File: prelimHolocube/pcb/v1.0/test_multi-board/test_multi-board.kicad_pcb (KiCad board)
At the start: 2 copper layers, 120 x 100 mm, 4 parts

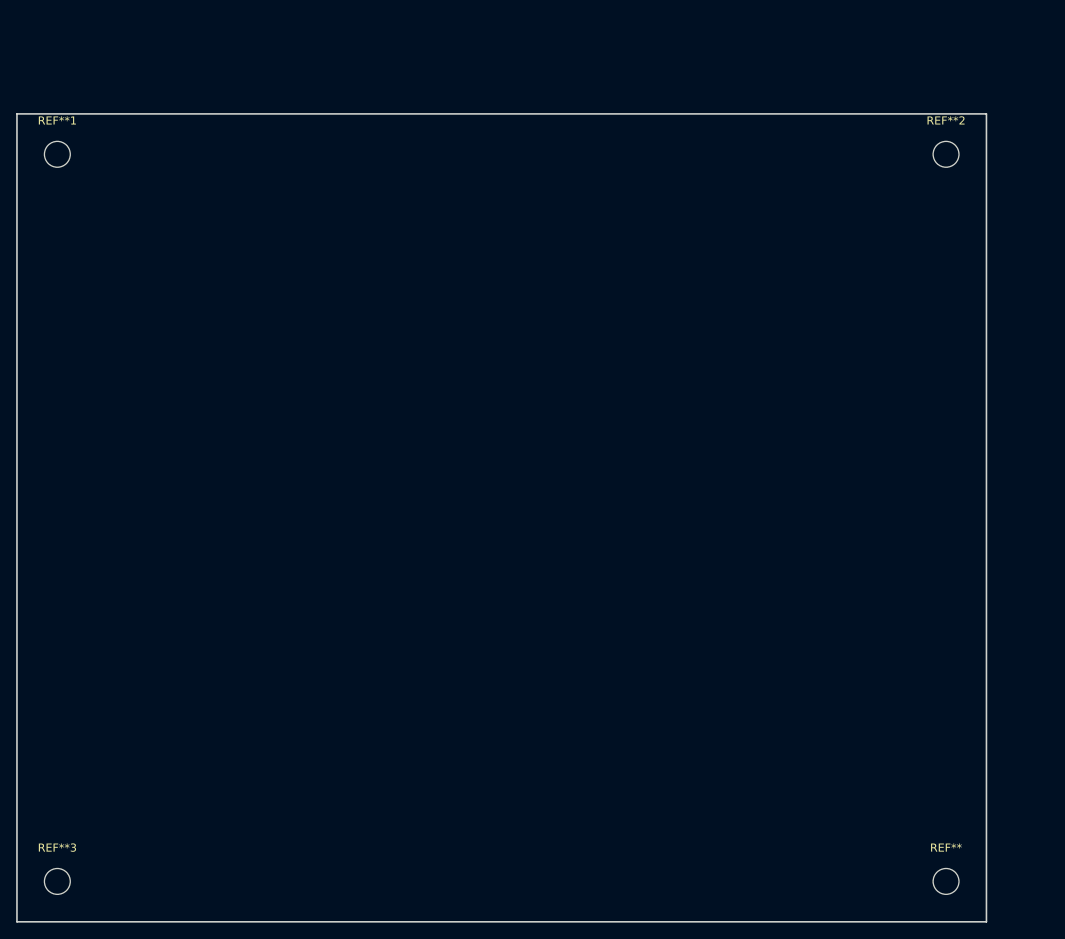
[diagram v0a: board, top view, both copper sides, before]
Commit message: Finish multiboard pcb
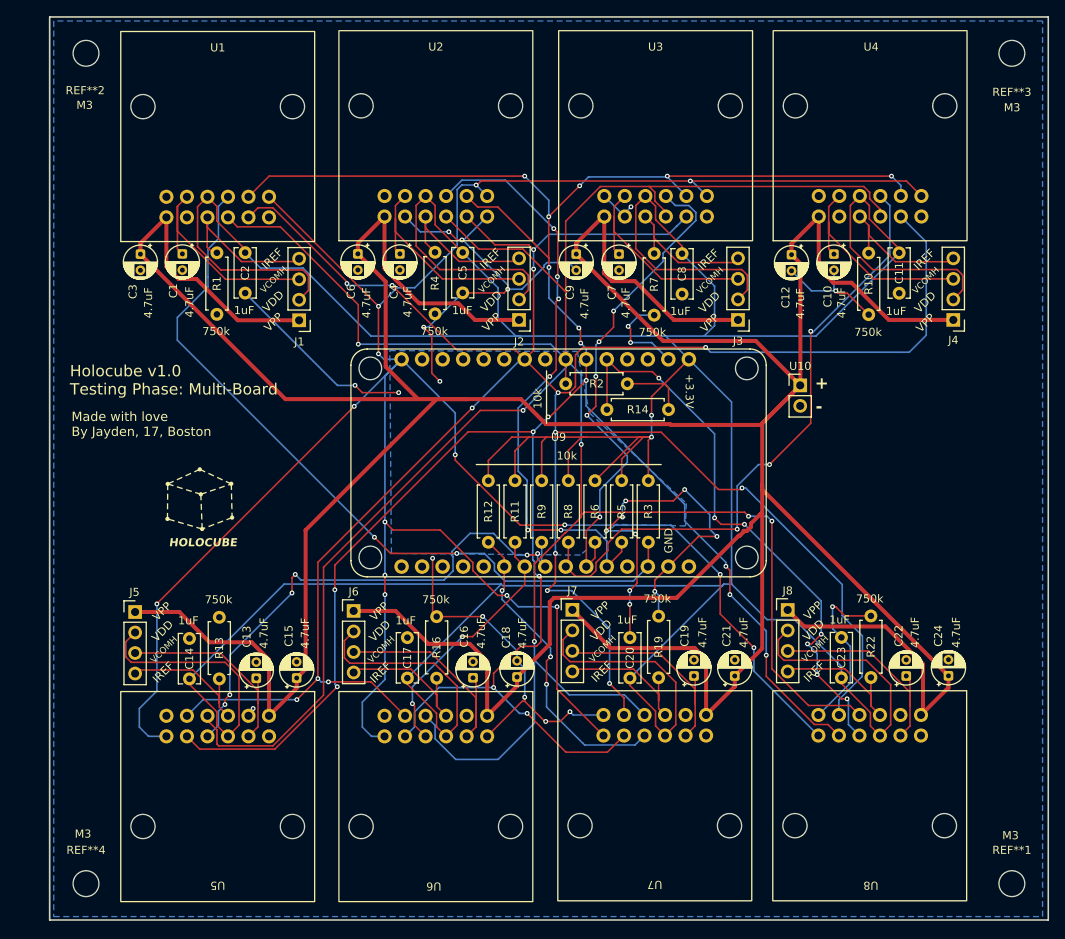
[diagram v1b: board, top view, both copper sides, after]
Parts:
- removed REF**: MountingHole_3.2mm_M3, MountingHole:MountingHole_3.2mm_M3
- added C1: 4.7uF, Capacitor_THT:CP_Radial_D4.0mm_P2.00mm, F.Cu at (109.9, 69.6)
- added C10: 4.7uF, Capacitor_THT:CP_Radial_D4.0mm_P2.00mm, F.Cu at (190.6, 69.7)
- added C11: 1uF ceramic, Capacitor_THT:C_Disc_D6.0mm_W2.5mm_P5.00mm, F.Cu at (198.7, 74.5)
- added C12: 4.7uF, Capacitor_THT:CP_Radial_D4.0mm_P2.00mm, F.Cu at (185.3, 69.7)
- added C13: 4.7uF, Capacitor_THT:CP_Radial_D4.0mm_P2.00mm, F.Cu at (119.1, 122.2)
- added C14: 1uF ceramic, Capacitor_THT:C_Disc_D6.0mm_W2.5mm_P5.00mm, F.Cu at (110.8, 117.2)
- added C15: 4.7uF, Capacitor_THT:CP_Radial_D4.0mm_P2.00mm, F.Cu at (124.1, 122.1)
- added C16: 4.7uF, Capacitor_THT:CP_Radial_D4.0mm_P2.00mm, F.Cu at (145.9, 122.1)
- added C17: 1uF ceramic, Capacitor_THT:C_Disc_D6.0mm_W2.5mm_P5.00mm, F.Cu at (137.8, 117.1)
- added C18: 4.7uF, Capacitor_THT:CP_Radial_D4.0mm_P2.00mm, F.Cu at (151.3, 122.0)
- added C19: 4.7uF, Capacitor_THT:CP_Radial_D4.0mm_P2.00mm, F.Cu at (173.2, 121.9)
- added C2: 1uF ceramic, Capacitor_THT:C_Disc_D6.0mm_W2.5mm_P5.00mm, F.Cu at (117.7, 74.5)
- added C20: 1uF ceramic, Capacitor_THT:C_Disc_D6.0mm_W2.5mm_P5.00mm, F.Cu at (165.3, 117.1)
- added C21: 4.7uF, Capacitor_THT:CP_Radial_D4.0mm_P2.00mm, F.Cu at (178.3, 121.9)
- added C22: 4.7uF, Capacitor_THT:CP_Radial_D4.0mm_P2.00mm, F.Cu at (199.5, 121.9)
- added C23: 1uF ceramic, Capacitor_THT:C_Disc_D6.0mm_W2.5mm_P5.00mm, F.Cu at (191.5, 117.1)
- added C24: 4.7uF, Capacitor_THT:CP_Radial_D4.0mm_P2.00mm, F.Cu at (204.8, 121.8)
- added C3: 4.7uF, Capacitor_THT:CP_Radial_D4.0mm_P2.00mm, F.Cu at (104.7, 69.7)
- added C4: 4.7uF, Capacitor_THT:CP_Radial_D4.0mm_P2.00mm, F.Cu at (136.8, 69.6)
- added C5: 1uF ceramic, Capacitor_THT:C_Disc_D6.0mm_W2.5mm_P5.00mm, F.Cu at (144.6, 74.5)
- added C6: 4.7uF, Capacitor_THT:CP_Radial_D4.0mm_P2.00mm, F.Cu at (131.7, 69.6)
- added C7: 4.7uF, Capacitor_THT:CP_Radial_D4.0mm_P2.00mm, F.Cu at (164.0, 69.7)
- added C8: 1uF ceramic, Capacitor_THT:C_Disc_D6.0mm_W2.5mm_P5.00mm, F.Cu at (171.8, 74.6)
- added C9: 4.7uF, Capacitor_THT:CP_Radial_D4.0mm_P2.00mm, F.Cu at (158.7, 69.7)
- added J1: Breakout_1, Connector_PinHeader_2.54mm:PinHeader_1x04_P2.54mm_Vertical, F.Cu at (124.4, 77.8)
- added J2: Breakout_2, Connector_PinHeader_2.54mm:PinHeader_1x04_P2.54mm_Vertical, F.Cu at (151.6, 77.8)
- added J3: Breakout_3, Connector_PinHeader_2.54mm:PinHeader_1x04_P2.54mm_Vertical, F.Cu at (178.7, 77.8)
- added J4: Breakout_4, Connector_PinHeader_2.54mm:PinHeader_1x04_P2.54mm_Vertical, F.Cu at (205.3, 77.8)
- added J5: Breakout_5, Connector_PinHeader_2.54mm:PinHeader_1x04_P2.54mm_Vertical, F.Cu at (104.1, 114.0)
- added J6: Breakout_6, Connector_PinHeader_2.54mm:PinHeader_1x04_P2.54mm_Vertical, F.Cu at (131.1, 113.8)
- added J7: Breakout_7, Connector_PinHeader_2.54mm:PinHeader_1x04_P2.54mm_Vertical, F.Cu at (158.2, 113.7)
- added J8: Breakout_8, Connector_PinHeader_2.54mm:PinHeader_1x04_P2.54mm_Vertical, F.Cu at (184.8, 113.7)
- added R1: 750k, Resistor_THT:R_Axial_DIN0207_L6.3mm_D2.5mm_P7.62mm_Horizontal, F.Cu at (114.2, 77.1)
- added R10: 750k, Resistor_THT:R_Axial_DIN0207_L6.3mm_D2.5mm_P7.62mm_Horizontal, F.Cu at (194.9, 77.1)
- added R11: 10k, Resistor_THT:R_Axial_DIN0207_L6.3mm_D2.5mm_P7.62mm_Horizontal, F.Cu at (151.1, 105.3)
- added R12: 10k, Resistor_THT:R_Axial_DIN0207_L6.3mm_D2.5mm_P7.62mm_Horizontal, F.Cu at (147.8, 105.3)
- added R13: 750k, Resistor_THT:R_Axial_DIN0207_L6.3mm_D2.5mm_P7.62mm_Horizontal, F.Cu at (114.5, 114.6)
- added R14: 10k, Resistor_THT:R_Axial_DIN0207_L6.3mm_D2.5mm_P7.62mm_Horizontal, F.Cu at (162.5, 88.9)
- added R16: 750k, Resistor_THT:R_Axial_DIN0207_L6.3mm_D2.5mm_P7.62mm_Horizontal, F.Cu at (141.4, 114.5)
- added R19: 750k, Resistor_THT:R_Axial_DIN0207_L6.3mm_D2.5mm_P7.62mm_Horizontal, F.Cu at (168.9, 114.5)
- added R2: 10k, Resistor_THT:R_Axial_DIN0207_L6.3mm_D2.5mm_P7.62mm_Horizontal, F.Cu at (157.4, 85.7)
- added R22: 750k, Resistor_THT:R_Axial_DIN0207_L6.3mm_D2.5mm_P7.62mm_Horizontal, F.Cu at (195.2, 114.4)
- added R3: 10k, Resistor_THT:R_Axial_DIN0207_L6.3mm_D2.5mm_P7.62mm_Horizontal, F.Cu at (167.6, 105.3)
- added R4: 750k, Resistor_THT:R_Axial_DIN0207_L6.3mm_D2.5mm_P7.62mm_Horizontal, F.Cu at (141.2, 77.0)
- added R5: 10k, Resistor_THT:R_Axial_DIN0207_L6.3mm_D2.5mm_P7.62mm_Horizontal, F.Cu at (164.3, 105.3)
- added R6: 10k, Resistor_THT:R_Axial_DIN0207_L6.3mm_D2.5mm_P7.62mm_Horizontal, F.Cu at (161.0, 105.3)
- added R7: 750k, Resistor_THT:R_Axial_DIN0207_L6.3mm_D2.5mm_P7.62mm_Horizontal, F.Cu at (168.3, 77.2)
- added R8: 10k, Resistor_THT:R_Axial_DIN0207_L6.3mm_D2.5mm_P7.62mm_Horizontal, F.Cu at (157.7, 105.3)
- added R9: 10k, Resistor_THT:R_Axial_DIN0207_L6.3mm_D2.5mm_P7.62mm_Horizontal, F.Cu at (154.4, 105.3)
- added REF**4: MountingHole_3.2mm_M3, MountingHole:MountingHole_3.2mm_M3, F.Cu at (98.0, 147.6)
- added U1: ~, transparent_oled_display:surenoo-1.12in-128x128, F.Cu at (114.3, 55.1)
- added U10: ~, Connector_PinHeader_2.54mm:PinHeader_1x02_P2.54mm_Vertical, F.Cu at (186.4, 85.9)
- added U2: ~, transparent_oled_display:surenoo-1.12in-128x128, F.Cu at (141.3, 55.0)
- added U3: ~, transparent_oled_display:surenoo-1.12in-128x128, F.Cu at (168.5, 55.0)
- added U4: ~, transparent_oled_display:surenoo-1.12in-128x128, F.Cu at (195.1, 55.0)
- added U5: ~, transparent_oled_display:surenoo-1.12in-128x128, F.Cu at (114.3, 136.8)
- added U6: ~, transparent_oled_display:surenoo-1.12in-128x128, F.Cu at (141.3, 136.8)
- added U7: ~, transparent_oled_display:surenoo-1.12in-128x128, F.Cu at (168.4, 136.7)
- added U8: ~, transparent_oled_display:surenoo-1.12in-128x128, F.Cu at (195.0, 136.7)
- added U9: ~, esp32:devkitv1-30pin, F.Cu at (156.5, 95.5)
- moved REF**3 156.4 mm to (212.6, 44.8)
- moved REF**1 148.7 mm to (212.6, 147.6)
- moved REF**2 107.2 mm to (98.0, 44.8)
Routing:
- net VDD_1: track 0.00 -> 636.2 mm, vias 0 -> 2
- net VPP_1: track 0.00 -> 580.8 mm
- net RES: track 0.00 -> 354.6 mm, vias 0 -> 6
- net SCL: track 0.00 -> 349.6 mm, vias 0 -> 15
- net SI: track 0.00 -> 348.4 mm, vias 0 -> 15
- net A0: track 0.00 -> 334.8 mm, vias 0 -> 19
- net GND: track 0.00 -> 224.8 mm, vias 0 -> 27
- net CS_1: track 0.00 -> 95.2 mm, vias 0 -> 2
- net CS_4: track 0.00 -> 79.2 mm, vias 0 -> 3
- net CS_2: track 0.00 -> 74.2 mm, vias 0 -> 6
- net CS_8: track 0.00 -> 72.0 mm, vias 0 -> 7
- net CS_5: track 0.00 -> 65.2 mm, vias 0 -> 6
- net CS_3: track 0.00 -> 61.6 mm, vias 0 -> 5
- net CS_7: track 0.00 -> 38.6 mm, vias 0 -> 3
- net CS_6: track 0.00 -> 31.7 mm, vias 0 -> 2
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- added copper zone on B.Cu, net GND
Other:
- board size 120 x 100 mm -> 123.6 x 111.8 mm
- board text added: "+"
- board text added: "+3.3V"
- board text added: "-"
- board text added: "10k"
- board text added: "1uF"
- board text added: "4.7uF"
- board text added: "750k"
- board text added: "GND"
- board text added: "HOLOCUBE"
- board text added: "Holocube v1.0 Testing Phase: Multi-Board"
- board text added: "IREF"
- board text added: "M3"
- board text added: "Made with love By Jayden, 17, Boston"
- board text added: "VCOMH"
- board text added: "VDD"
- board text added: "VPP"
